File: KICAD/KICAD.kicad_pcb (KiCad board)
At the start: 2 copper layers, 266 parts, among them J11 Conn_01x04_Pin, J4 Conn_01x03_Pin, J5 Conn_01x03_Pin, U1 CD4066BE, U2 CD4066BE, U3 CD4066BE, U4 CD4066BE

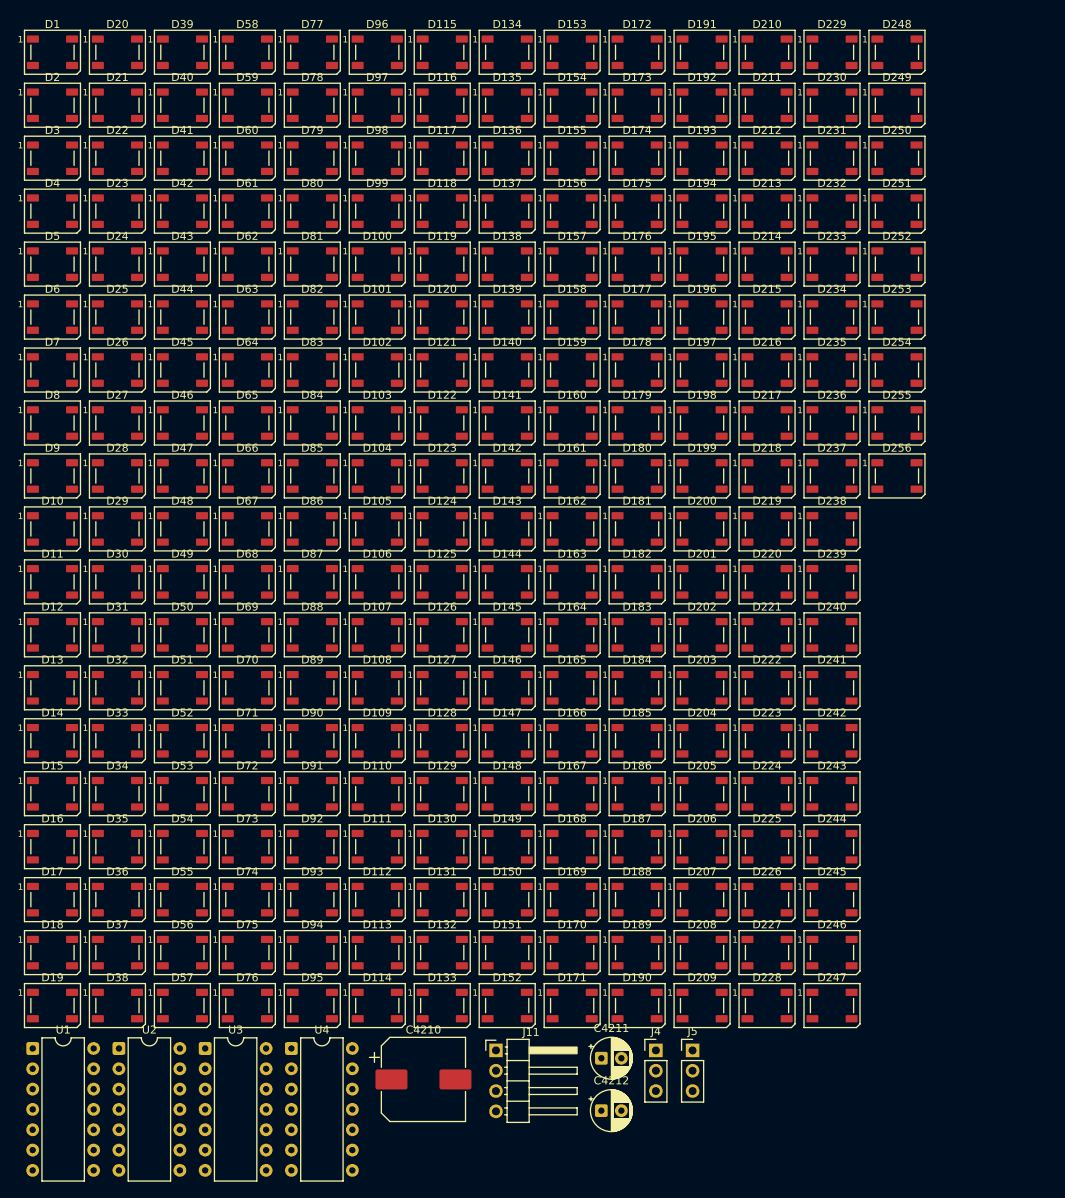
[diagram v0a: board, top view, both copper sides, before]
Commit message: .
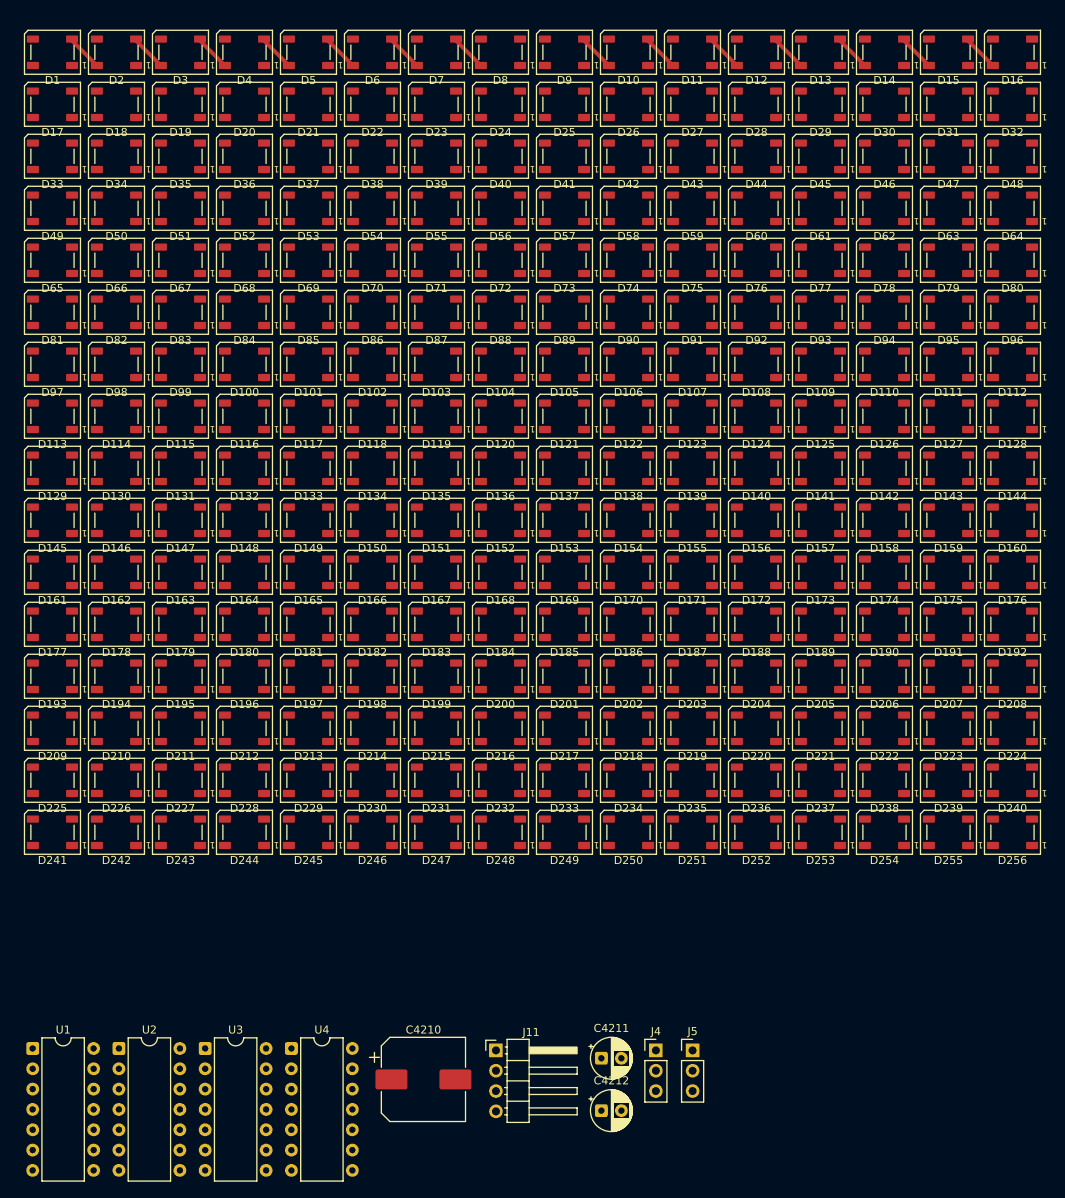
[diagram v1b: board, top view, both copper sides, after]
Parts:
- moved D16 155.8 mm to (641.5, 268.8), turned to 180 degrees
- moved D15 145.4 mm to (633.5, 268.8), turned to 180 degrees
- moved D14 135.0 mm to (625.5, 268.8), turned to 180 degrees
- moved D32 133.6 mm to (641.5, 275.3), turned to 180 degrees
- moved D13 124.6 mm to (617.5, 268.8), turned to 180 degrees
- moved D31 123.2 mm to (633.5, 275.3), turned to 180 degrees
- moved D95 117.6 mm to (633.5, 301.3), turned to 180 degrees
- moved D210 117.3 mm to (529.5, 353.3), turned to 180 degrees
- moved D12 114.2 mm to (609.5, 268.8), turned to 180 degrees
- moved D19 113.8 mm to (537.5, 275.3), turned to 180 degrees
- moved D48 113.7 mm to (641.5, 281.8), turned to 180 degrees
- moved D30 112.9 mm to (625.5, 275.3), turned to 180 degrees
- moved D76 112.8 mm to (609.5, 294.8), turned to 180 degrees
- moved D229 112.1 mm to (553.5, 359.8), turned to 180 degrees
- moved D38 110.8 mm to (561.5, 281.8), turned to 180 degrees
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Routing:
- net Net-(D7-DOUT): track 0.00 -> 4.58 mm
- net Net-(D6-DOUT): track 0.00 -> 4.58 mm
- net Net-(D5-DOUT): track 0.00 -> 4.58 mm
- net Net-(D4-DOUT): track 0.00 -> 4.58 mm
- net Net-(D3-DOUT): track 0.00 -> 4.58 mm
- net Net-(D2-DOUT): track 0.00 -> 4.58 mm
- net Net-(D15-DOUT): track 0.00 -> 4.58 mm
- net Net-(D14-DOUT): track 0.00 -> 4.58 mm
- net Net-(D13-DOUT): track 0.00 -> 4.58 mm
- net Net-(D12-DOUT): track 0.00 -> 4.58 mm
- net Net-(D11-DOUT): track 0.00 -> 4.58 mm
- net Net-(D10-DOUT): track 0.00 -> 4.58 mm
- net Net-(D10-DIN): track 0.00 -> 4.58 mm
- net Net-(D1-DOUT): track 0.00 -> 4.58 mm
